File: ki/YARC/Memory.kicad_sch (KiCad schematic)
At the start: 18 parts, among them U14 74LS20, U18 AS6C6264, U20 74HC00, U21 74LS08, U22 74LS139, U23 74LS32, U24 AS6C6264, U25 74HC245, U26 74LS157, U27 AS6C6264, U28 74HC245, U29 AS6C6264, U30 74HC245

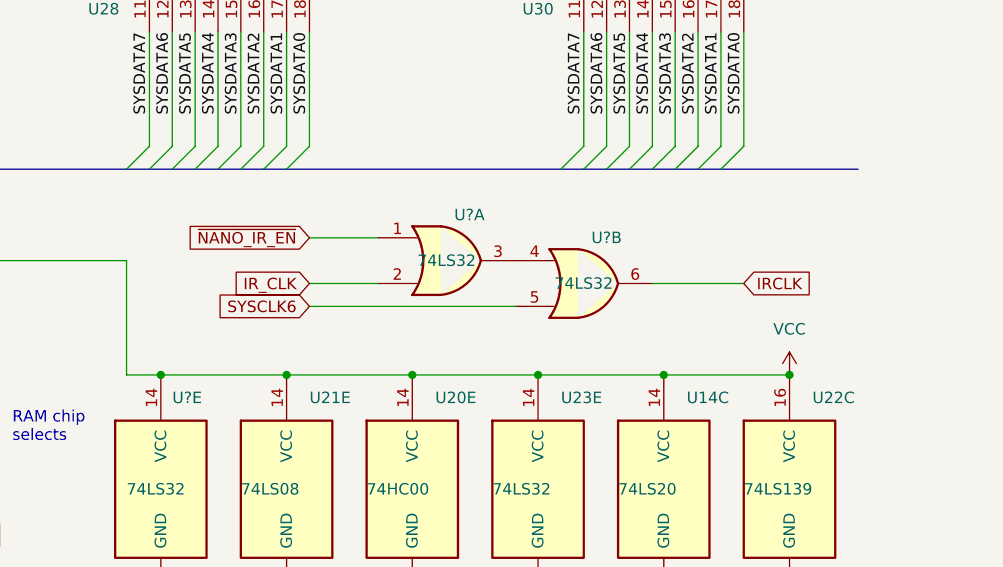
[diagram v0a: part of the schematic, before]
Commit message: Continuing work on microcode control
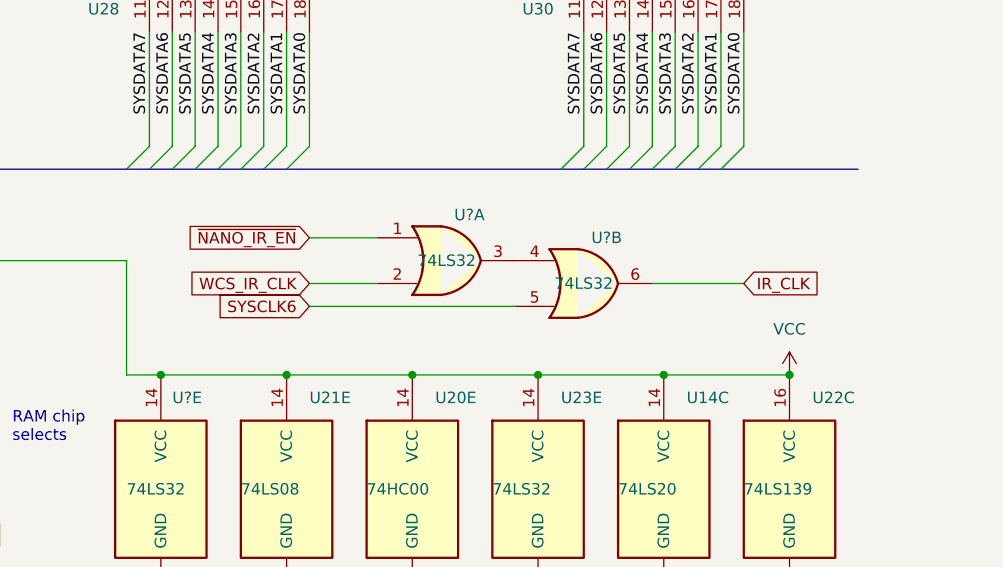
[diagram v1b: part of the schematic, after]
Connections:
- net IRCLK is gone; now on net IR_CLK: U?.6
- net IR_CLK: no longer U?.2
- new net WCS_IR_CLK: U?.2
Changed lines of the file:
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@@
     )
   )
-  (global_label "IR_CLK" (shape input) (at 203.2 134.62 180) (fields_autoplaced)
+  (global_label "WCS_IR_CLK" (shape input) (at 203.2 134.62 180) (fields_autoplaced)
     (effects (font (size 1.27 1.27)) (justify right))
-    (property "Intersheet References" "${INTERSHEET_REFS}" (id 0) (at 194.3764 134.5406 0)
+    (property "Intersheet References" "${INTERSHEET_REFS}" (id 0) (at 189.4779 134.5406 0)
       (effects (font (size 1.27 1.27)) (justify right) hide)
     )
@@
     )
   )
-  (global_label "IRCLK" (shape input) (at 251.46 134.62 0) (fields_autoplaced)
+  (global_label "IR_CLK" (shape input) (at 251.46 134.62 0) (fields_autoplaced)
     (effects (font (size 1.27 1.27)) (justify left))
-    (property "Intersheet References" "${INTERSHEET_REFS}" (id 0) (at 259.316 134.5406 0)
+    (property "Intersheet References" "${INTERSHEET_REFS}" (id 0) (at 260.2836 134.5406 0)
       (effects (font (size 1.27 1.27)) (justify left) hide)
     )
